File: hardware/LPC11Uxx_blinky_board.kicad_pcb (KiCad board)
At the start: 2 copper layers, 20 x 40 mm, 23 parts, among them J1 Conn_ARM_JTAG_SWD_10, J2 USB_B_Micro, J3 Conn_01x04_Male, SW1 SW_Push, U1 LPC11U37FBD48-401_, U2 MCP1825S, Y1 Crystal

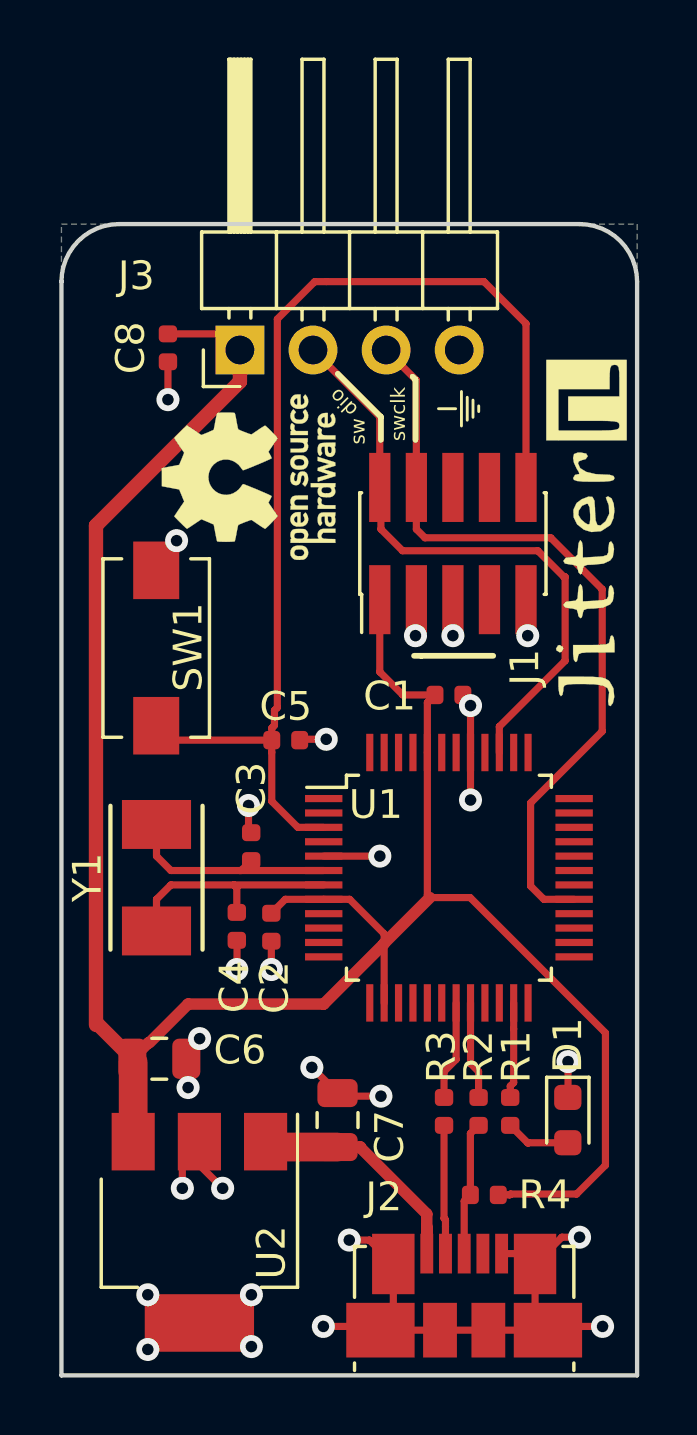
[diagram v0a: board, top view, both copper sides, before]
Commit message: PCB layout: minor adjustments
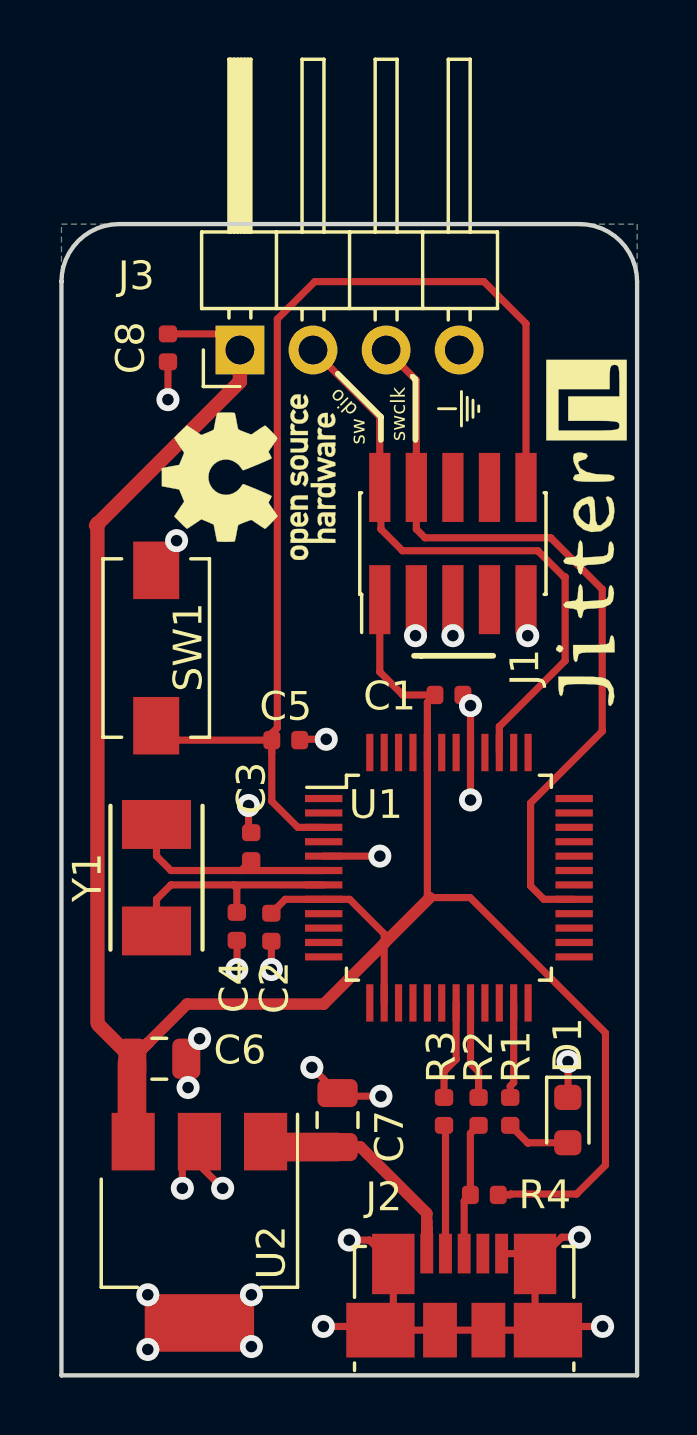
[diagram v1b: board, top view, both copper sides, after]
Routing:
- net +3V3: track 81.9 -> 82.7 mm
- net +5V: track 8.25 -> 8.97 mm
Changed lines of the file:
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@@
-(kicad_pcb (version 20171130) (host pcbnew "(5.0.1-3-g963ef8bb5)")
+(kicad_pcb (version 20171130) (host pcbnew 5.0.1-33cea8e~68~ubuntu18.04.1)
   (general
     (thickness 1.6)
     (drawings 35)
-    (tracks 194)
+    (tracks 188)
     (zones 0)
     (modules 23)
@@
     (34 B.Paste user hide)
     (35 F.Paste user hide)
-    (36 B.SilkS user hide)
-    (37 F.SilkS user hide)
+    (36 B.SilkS user)
+    (37 F.SilkS user)
     (38 B.Mask user hide)
     (39 F.Mask user)
@@
   (via (at 33.6 34.1) (size 0.8) (drill 0.4) (layers F.Cu B.Cu) (net 1))
   (segment (start 33.6 32.85) (end 33.6 34.1) (width 0.25) (layer F.Cu) (net 1))
-  (segment (start 29.112498 46.9) (end 31.212498 44.8) (width 0.4) (layer F.Cu) (net 2))
   (segment (start 22.492498 48.929998) (end 22.3625 48.8) (width 0.25) (layer F.Cu) (net 2))
   (segment (start 35.177498 53.530002) (end 35.572498 53.530002) (width 0.25) (layer F.Cu) (net 2))
@@
   (segment (start 31.860002 36.160002) (end 32.977498 36.160002) (width 0.25) (layer F.Cu) (net 2))
   (segment (start 31.212498 44.8) (end 31.212498 46.860002) (width 0.25) (layer F.Cu) (net 2))
-  (segment (start 23.056237 48.243763) (end 24.4 46.9) (width 0.4) (layer F.Cu) (net 2))
-  (segment (start 24.4 46.9) (end 29.112498 46.9) (width 0.4) (layer F.Cu) (net 2))
   (segment (start 22.4625 48.8) (end 23.018737 48.243763) (width 0.4) (layer F.Cu) (net 2))
   (segment (start 23.018737 48.243763) (end 23.056237 48.243763) (width 0.25) (layer F.Cu) (net 2))
-  (segment (start 22.492498 51.680002) (end 22.492498 48.929998) (width 1) (layer F.Cu) (net 2))
+  (segment (start 22.45 51.700004) (end 22.45 48.95) (width 1) (layer F.Cu) (net 2))
   (segment (start 38.9 47.9) (end 34.2 43.2) (width 0.25) (layer F.Cu) (net 2))
   (segment (start 34.2 43.2) (end 32.8 43.2) (width 0.25) (layer F.Cu) (net 2))
@@
   (segment (start 21.287504 47.625004) (end 22.4625 48.8) (width 0.5) (layer F.Cu) (net 2))
   (segment (start 26.2 25.275) (end 21.2 30.275) (width 0.5) (layer F.Cu) (net 2))
-  (segment (start 21.2 30.275) (end 21.2 47.625004) (width 0.5) (layer F.Cu) (net 2) (status 40000))
   (segment (start 31.06 35.36) (end 31.860002 36.160002) (width 0.25) (layer F.Cu) (net 2))
   (segment (start 31.06 32.85) (end 31.06 35.36) (width 0.25) (layer F.Cu) (net 2))
@@
   (segment (start 30.012498 43.260002) (end 31.212498 44.460002) (width 0.25) (layer F.Cu) (net 2))
   (segment (start 31.212498 44.460002) (end 31.212498 44.8) (width 0.25) (layer F.Cu) (net 2))
+  (segment (start 21.25 30.199996) (end 21.25 47.55) (width 0.5) (layer F.Cu) (net 2) (status 40000))
+  (segment (start 24.3625 46.9) (end 22.4625 48.8) (width 0.4) (layer F.Cu) (net 2))
+  (segment (start 31.212498 44.8) (end 29.112498 46.9) (width 0.4) (layer F.Cu) (net 2))
+  (segment (start 29.112498 46.9) (end 24.3625 46.9) (width 0.4) (layer F.Cu) (net 2))
   (segment (start 26.247498 42.260002) (end 26.192498 42.260002) (width 0.25) (layer F.Cu) (net 3))
   (segment (start 29.112498 42.260002) (end 26.192498 42.260002) (width 0.25) (layer F.Cu) (net 3))
@@
   (segment (start 28.212498 40.760002) (end 27.307498 39.855002) (width 0.25) (layer F.Cu) (net 5))
   (segment (start 27.307498 37.730002) (end 23.792498 37.730002) (width 0.25) (layer F.Cu) (net 5))
+  (segment (start 36.14 23.26) (end 34.68 21.8) (width 0.25) (layer F.Cu) (net 5))
+  (segment (start 28.8 21.8) (end 27.5 23.1) (width 0.25) (layer F.Cu) (net 5))
   (segment (start 36.14 28.95) (end 36.14 23.26) (width 0.25) (layer F.Cu) (net 5))
-  (segment (start 36.14 23.26) (end 34.68 21.8) (width 0.25) (layer F.Cu) (net 5))
-  (segment (start 34.68 21.8) (end 29.2 21.8) (width 0.25) (layer F.Cu) (net 5))
-  (segment (start 28.8 21.8) (end 29.2 21.8) (width 0.25) (layer F.Cu) (net 5))
-  (segment (start 27.5 23.1) (end 28.8 21.8) (width 0.25) (layer F.Cu) (net 5))
-  (segment (start 27.4 36.7) (end 27.5 36.6) (width 0.25) (layer F.Cu) (net 5))
-  (segment (start 27.5 36.6) (end 27.5 23.1) (width 0.25) (layer F.Cu) (net 5))
-  (segment (start 27.4 37.2175) (end 27.4 36.7) (width 0.25) (layer F.Cu) (net 5))
-  (segment (start 27.307498 37.310002) (end 27.4 37.2175) (width 0.25) (layer F.Cu) (net 5))
-  (segment (start 27.307498 37.730002) (end 27.307498 37.310002) (width 0.25) (layer F.Cu) (net 5))
+  (segment (start 34.68 21.8) (end 28.8 21.8) (width 0.25) (layer F.Cu) (net 5))
+  (segment (start 27.307498 37.492502) (end 27.307498 37.730002) (width 0.25) (layer F.Cu) (net 5))
+  (segment (start 27.5 23.1) (end 27.5 37.3) (width 0.25) (layer F.Cu) (net 5))
+  (segment (start 27.5 37.3) (end 27.307498 37.492502) (width 0.25) (layer F.Cu) (net 5))
   (segment (start 27.279998 51.867502) (end 27.092498 51.680002) (width 0.25) (layer F.Cu) (net 6))
-  (segment (start 30.392498 51.867502) (end 30.392498 51.892498) (width 0.4) (layer F.Cu) (net 6))
   (segment (start 32.692498 55.570002) (end 32.692498 54.85) (width 0.4) (layer F.Cu) (net 6))
   (segment (start 32.692498 54.85) (end 32.692498 54.630002) (width 0.4) (layer F.Cu) (net 6))
-  (segment (start 30.392498 51.892498) (end 32.692498 54.192498) (width 0.4) (layer F.Cu) (net 6))
   (segment (start 29.592498 51.867502) (end 27.279998 51.867502) (width 1) (layer F.Cu) (net 6))
+  (segment (start 32.692498 54.480002) (end 32.692498 55.570002) (width 0.4) (layer F.Cu) (net 6))
+  (segment (start 32.692498 54.167502) (end 32.692498 54.480002) (width 0.4) (layer F.Cu) (net 6))
+  (segment (start 30.392498 51.867502) (end 32.692498 54.167502) (width 0.4) (layer F.Cu) (net 6))
   (segment (start 29.592498 51.867502) (end 30.392498 51.867502) (width 0.4) (layer F.Cu) (net 6))
-  (segment (start 32.692498 54.192498) (end 32.692498 54.85) (width 0.4) (layer F.Cu) (net 6))
   (segment (start 36.207498 51.730002) (end 36.219998 51.717502) (width 0.25) (layer F.Cu) (net 7))
   (segment (start 36.219998 51.717502) (end 37.592498 51.717502) (width 0.25) (layer F.Cu) (net 7))
@@
   (segment (start 34.207498 51.400002) (end 34.492498 51.115002) (width 0.25) (layer F.Cu) (net 14))
   (segment (start 34.207498 53.530002) (end 34.207498 51.400002) (width 0.25) (layer F.Cu) (net 14))
-  (segment (start 33.292498 51.115002) (end 33.292498 54.346106) (width 0.25) (layer F.Cu) (net 15))
-  (segment (start 33.342498 54.396106) (end 33.342498 54.630002) (width 0.25) (layer F.Cu) (net 15))
-  (segment (start 33.342498 54.630002) (end 33.342498 55.570002) (width 0.25) (layer F.Cu) (net 15))
   (segment (start 33.342498 51.165002) (end 33.292498 51.115002) (width 0.25) (layer F.Cu) (net 15))
-  (segment (start 33.292498 54.346106) (end 33.342498 54.396106) (width 0.25) (layer F.Cu) (net 15))
+  (segment (start 33.342498 51.165002) (end 33.342498 55.570002) (width 0.25) (layer F.Cu) (net 15))
   (segment (start 35.592498 50.145002) (end 35.592498 49.750002) (width 0.25) (layer F.Cu) (net 16))
   (segment (start 35.712498 47.760002) (end 35.712498 46.860002) (width 0.25) (layer F.Cu) (net 16))
@@
     (connect_pads (clearance 0.508))
     (min_thickness 0.254)
-    (fill yes (arc_segments 16) (thermal_gap 0.508) (thermal_bridge_width 0.508))
+    (fill yes (arc_segments 32) (thermal_gap 0.508) (thermal_bridge_width 0.508))
     (polygon
       (pts
